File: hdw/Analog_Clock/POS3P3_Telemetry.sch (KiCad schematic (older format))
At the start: 11 parts

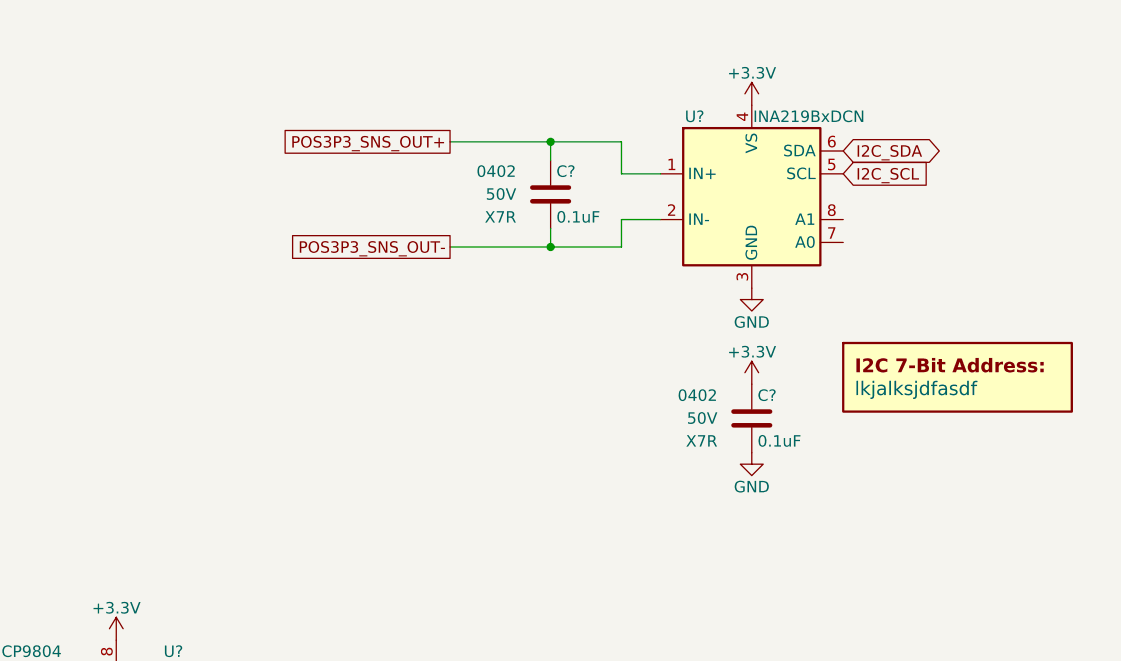
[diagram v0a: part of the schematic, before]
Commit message: More schematic work
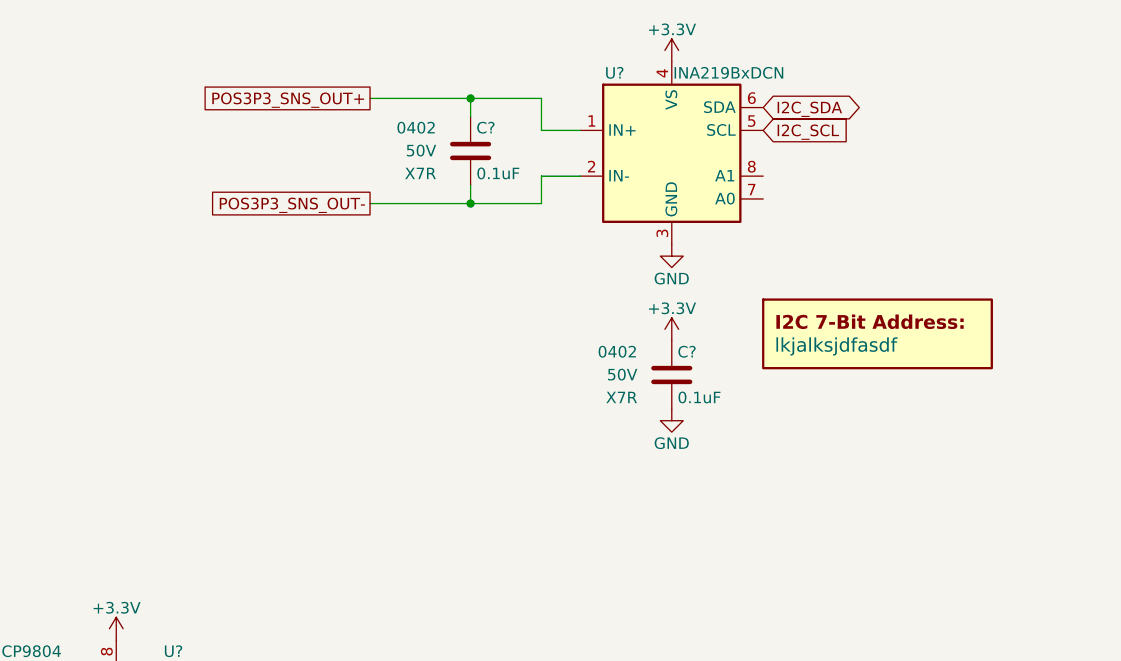
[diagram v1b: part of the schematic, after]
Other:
- moved on the sheet: C?, U?
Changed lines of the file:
@@
 EESchema Schematic File Version 4
+LIBS:Analog_Clock-cache
 EELAYER 30 0
 EELAYER END
@@
 	1    0    0    -1
 $EndComp
-Text GLabel 6890 2160 0    50   UnSpc ~ 0
+Text GLabel 6540 1970 0    50   UnSpc ~ 0
 POS3P3_SNS_OUT+
-Text GLabel 6890 2620 0    50   UnSpc ~ 0
+Text GLabel 6540 2430 0    50   UnSpc ~ 0
 POS3P3_SNS_OUT-
 $Comp
@@
 L power:GND #PWR?
 U 1 1 5E1C292F
-P 8210 2800
+P 7860 2610
 AR Path="/5E0652BA/5E1C292F" Ref="#PWR?"  Part="1"
 AR Path="/5E0A0E29/5E1C292F" Ref="#PWR?"  Part="1"
 AR Path="/5E052856/5E1C292F" Ref="#PWR?"  Part="1"
 AR Path="/5E939D42/5E1C292F" Ref="#PWR?"  Part="1"
-F 0 "#PWR?" H 8210 2550 50  0001 C CNN
-F 1 "GND" H 8210 2650 50  0000 C CNN
-F 2 "" H 8210 2800 50  0001 C CNN
-F 3 "" H 8210 2800 50  0001 C CNN
-	1    8210 2800
+F 0 "#PWR?" H 7860 2360 50  0001 C CNN
+F 1 "GND" H 7860 2460 50  0000 C CNN
+F 2 "" H 7860 2610 50  0001 C CNN
+F 3 "" H 7860 2610 50  0001 C CNN
+	1    7860 2610
 	1    0    0    -1
 $EndComp
@@
 L power:+3.3V #PWR?
 U 1 1 5E1C2935
-P 8210 2000
+P 7860 1810
 AR Path="/5E0652BA/5E1C2935" Ref="#PWR?"  Part="1"
 AR Path="/5E0A0E29/5E1C2935" Ref="#PWR?"  Part="1"
 AR Path="/5E052856/5E1C2935" Ref="#PWR?"  Part="1"
 AR Path="/5E939D42/5E1C2935" Ref="#PWR?"  Part="1"
-F 0 "#PWR?" H 8210 1850 50  0001 C CNN
-F 1 "+3.3V" H 8210 2140 50  0000 C CNN
-F 2 "" H 8210 2000 50  0001 C CNN
-F 3 "" H 8210 2000 50  0001 C CNN
-	1    8210 2000
-	1    0    0    -1
-$EndComp
-Text GLabel 8610 2300 2    50   Input ~ 0
+F 0 "#PWR?" H 7860 1660 50  0001 C CNN
+F 1 "+3.3V" H 7860 1950 50  0000 C CNN
+F 2 "" H 7860 1810 50  0001 C CNN
+F 3 "" H 7860 1810 50  0001 C CNN
+	1    7860 1810
+	1    0    0    -1
+$EndComp
+Text GLabel 8260 2110 2    50   Input ~ 0
 I2C_SCL
 $Comp
 L Custom_Library:C_Custom C?
 U 1 1 5E1C2940
-P 8210 3370
+P 7860 3180
 AR Path="/5B3E071A/5E1C2940" Ref="C?"  Part="1"
 AR Path="/5E0652BA/5E1C2940" Ref="C?"  Part="1"
@@
 AR Path="/5E052856/5E1C2940" Ref="C?"  Part="1"
 AR Path="/5E939D42/5E1C2940" Ref="C?"  Part="1"
-F 0 "C?" H 8235 3470 50  0000 L CNN
-F 1 "0.1uF" H 8235 3270 50  0000 L CNN
-F 2 "Capacitors_SMD:C_0402" H 8248 3220 50  0001 C CNN
-F 3 "" H 8235 3470 50  0001 C CNN
-F 4 "0402" H 8060 3470 50  0000 R CNN "display_footprint"
-F 5 "50V" H 8060 3370 50  0000 R CNN "Voltage"
-F 6 "X7R" H 8060 3270 50  0000 R CNN "Dielectric"
-F 7 "490-10701-1-ND" H 4300 -3510 50  0001 C CNN "Digi-Key PN"
-	1    8210 3370
+F 0 "C?" H 7885 3280 50  0000 L CNN
+F 1 "0.1uF" H 7885 3080 50  0000 L CNN
+F 2 "Capacitors_SMD:C_0402" H 7898 3030 50  0001 C CNN
+F 3 "" H 7885 3280 50  0001 C CNN
+F 4 "0402" H 7710 3280 50  0000 R CNN "display_footprint"
+F 5 "50V" H 7710 3180 50  0000 R CNN "Voltage"
+F 6 "X7R" H 7710 3080 50  0000 R CNN "Dielectric"
+F 7 "490-10701-1-ND" H 3950 -3700 50  0001 C CNN "Digi-Key PN"
+	1    7860 3180
 	1    0    0    -1
 $EndComp
@@
 L power:+3.3V #PWR?
 U 1 1 5E1C2946
-P 8210 3220
+P 7860 3030
 AR Path="/5E0652BA/5E1C2946" Ref="#PWR?"  Part="1"
 AR Path="/5E0A0E29/5E1C2946" Ref="#PWR?"  Part="1"
 AR Path="/5E052856/5E1C2946" Ref="#PWR?"  Part="1"
 AR Path="/5E939D42/5E1C2946" Ref="#PWR?"  Part="1"
-F 0 "#PWR?" H 8210 3070 50  0001 C CNN
-F 1 "+3.3V" H 8210 3360 50  0000 C CNN
-F 2 "" H 8210 3220 50  0001 C CNN
-F 3 "" H 8210 3220 50  0001 C CNN
-	1    8210 3220
+F 0 "#PWR?" H 7860 2880 50  0001 C CNN
+F 1 "+3.3V" H 7860 3170 50  0000 C CNN
+F 2 "" H 7860 3030 50  0001 C CNN
+F 3 "" H 7860 3030 50  0001 C CNN
+	1    7860 3030
 	1    0    0    -1
 $EndComp
@@
 L power:GND #PWR?
 U 1 1 5E1C294C
-P 8210 3520
+P 7860 3330
 AR Path="/5E0652BA/5E1C294C" Ref="#PWR?"  Part="1"
 AR Path="/5E0A0E29/5E1C294C" Ref="#PWR?"  Part="1"
 AR Path="/5E052856/5E1C294C" Ref="#PWR?"  Part="1"
 AR Path="/5E939D42/5E1C294C" Ref="#PWR?"  Part="1"
-F 0 "#PWR?" H 8210 3270 50  0001 C CNN
-F 1 "GND" H 8210 3370 50  0000 C CNN
-F 2 "" H 8210 3520 50  0001 C CNN
-F 3 "" H 8210 3520 50  0001 C CNN
-	1    8210 3520
-	1    0    0    -1
-$EndComp
-Text GLabel 8610 2200 2    50   BiDi ~ 0
+F 0 "#PWR?" H 7860 3080 50  0001 C CNN
+F 1 "GND" H 7860 3180 50  0000 C CNN
+F 2 "" H 7860 3330 50  0001 C CNN
+F 3 "" H 7860 3330 50  0001 C CNN
+	1    7860 3330
+	1    0    0    -1
+$EndComp
+Text GLabel 8260 2010 2    50   BiDi ~ 0
 I2C_SDA
 $Comp
 L Custom_Library:I2C_Address DOC?
 U 1 1 5E1C2953
-P 9110 3240
+P 8760 3050
 AR Path="/5E0652BA/5E1C2953" Ref="DOC?"  Part="1"
 AR Path="/5E0A0E29/5E1C2953" Ref="DOC?"  Part="1"
 AR Path="/5E052856/5E1C2953" Ref="DOC?"  Part="1"
 AR Path="/5E939D42/5E1C2953" Ref="DOC?"  Part="1"
-F 0 "DOC?" H 9110 3490 60  0001 C CNN
-F 1 "lkjalksjdfasdf" H 8660 3240 60  0000 L CNN
-F 2 "" H 9110 3590 60  0001 C CNN
-F 3 "" H 9110 3590 60  0001 C CNN
-	1    9110 3240
-	1    0    0    -1
-$EndComp
-Wire Wire Line
-	7330 2620 7330 2540
-Wire Wire Line
-	7330 2240 7330 2160
+F 0 "DOC?" H 8760 3300 60  0001 C CNN
+F 1 "lkjalksjdfasdf" H 8310 3050 60  0000 L CNN
+F 2 "" H 8760 3400 60  0001 C CNN
+F 3 "" H 8760 3400 60  0001 C CNN
+	1    8760 3050
+	1    0    0    -1
+$EndComp
+Wire Wire Line
+	6980 2430 6980 2350
+Wire Wire Line
+	6980 2050 6980 1970
 $Comp
 L Custom_Library:C_Custom C?
 U 1 1 5E1C295F
-P 7330 2390
+P 6980 2200
 AR Path="/5B3E071A/5E1C295F" Ref="C?"  Part="1"
 AR Path="/5E0652BA/5E1C295F" Ref="C?"  Part="1"
@@
 AR Path="/5E052856/5E1C295F" Ref="C?"  Part="1"
 AR Path="/5E939D42/5E1C295F" Ref="C?"  Part="1"
-F 0 "C?" H 7355 2490 50  0000 L CNN
-F 1 "0.1uF" H 7355 2290 50  0000 L CNN
-F 2 "Capacitors_SMD:C_0402" H 7368 2240 50  0001 C CNN
-F 3 "" H 7355 2490 50  0001 C CNN
-F 4 "0402" H 7180 2490 50  0000 R CNN "display_footprint"
-F 5 "50V" H 7180 2390 50  0000 R CNN "Voltage"
-F 6 "X7R" H 7180 2290 50  0000 R CNN "Dielectric"
-F 7 "490-10701-1-ND" H 3420 -4490 50  0001 C CNN "Digi-Key PN"
-	1    7330 2390
-	1    0    0    -1
-$EndComp
-Wire Wire Line
-	6890 2620 7330 2620
-Wire Wire Line
-	6890 2160 7330 2160
+F 0 "C?" H 7005 2300 50  0000 L CNN
+F 1 "0.1uF" H 7005 2100 50  0000 L CNN
+F 2 "Capacitors_SMD:C_0402" H 7018 2050 50  0001 C CNN
+F 3 "" H 7005 2300 50  0001 C CNN
+F 4 "0402" H 6830 2300 50  0000 R CNN "display_footprint"
+F 5 "50V" H 6830 2200 50  0000 R CNN "Voltage"
+F 6 "X7R" H 6830 2100 50  0000 R CNN "Dielectric"
+F 7 "490-10701-1-ND" H 3070 -4680 50  0001 C CNN "Digi-Key PN"
+	1    6980 2200
+	1    0    0    -1
+$EndComp
+Wire Wire Line
+	6540 2430 6980 2430
+Wire Wire Line
+	6540 1970 6980 1970
 $Comp
 L Analog_ADC:INA219BxDCN U?
 U 1 1 5E1C297C
-P 8210 2400
-F 0 "U?" H 7960 2750 50  0000 C CNN
-F 1 "INA219BxDCN" H 8460 2750 50  0000 C CNN
-F 2 "Package_TO_SOT_SMD:SOT-23-8" H 8860 2050 50  0001 C CNN
-F 3 "http://www.ti.com/lit/ds/symlink/ina219.pdf" H 8560 2300 50  0001 C CNN
-F 4 "296-46420-1-ND" H 8210 2400 50  0001 C CNN "Digi-Key PN"
-	1    8210 2400
-	1    0    0    -1
-$EndComp
-Wire Wire Line
-	7810 2300 7640 2300
-Wire Wire Line
-	7640 2300 7640 2160
-Wire Wire Line
-	7640 2160 7330 2160
-Connection ~ 7330 2160
-Wire Wire Line
-	7810 2500 7640 2500
-Wire Wire Line
-	7640 2500 7640 2620
-Wire Wire Line
-	7640 2620 7330 2620
-Connection ~ 7330 2620
+P 7860 2210
+F 0 "U?" H 7610 2560 50  0000 C CNN
+F 1 "INA219BxDCN" H 8110 2560 50  0000 C CNN
+F 2 "Package_TO_SOT_SMD:SOT-23-8" H 8510 1860 50  0001 C CNN
+F 3 "http://www.ti.com/lit/ds/symlink/ina219.pdf" H 8210 2110 50  0001 C CNN
+F 4 "296-46420-1-ND" H 7860 2210 50  0001 C CNN "Digi-Key PN"
+	1    7860 2210
+	1    0    0    -1
+$EndComp
+Wire Wire Line
+	7460 2110 7290 2110
+Wire Wire Line
+	7290 2110 7290 1970
+Wire Wire Line
+	7290 1970 6980 1970
+Connection ~ 6980 1970
+Wire Wire Line
+	7460 2310 7290 2310
+Wire Wire Line
+	7290 2310 7290 2430
+Wire Wire Line
+	7290 2430 6980 2430
+Connection ~ 6980 2430
 $Comp
 L Analog_ADC:INA219BxDCN U?
